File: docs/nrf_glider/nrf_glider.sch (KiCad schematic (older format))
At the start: 26 parts

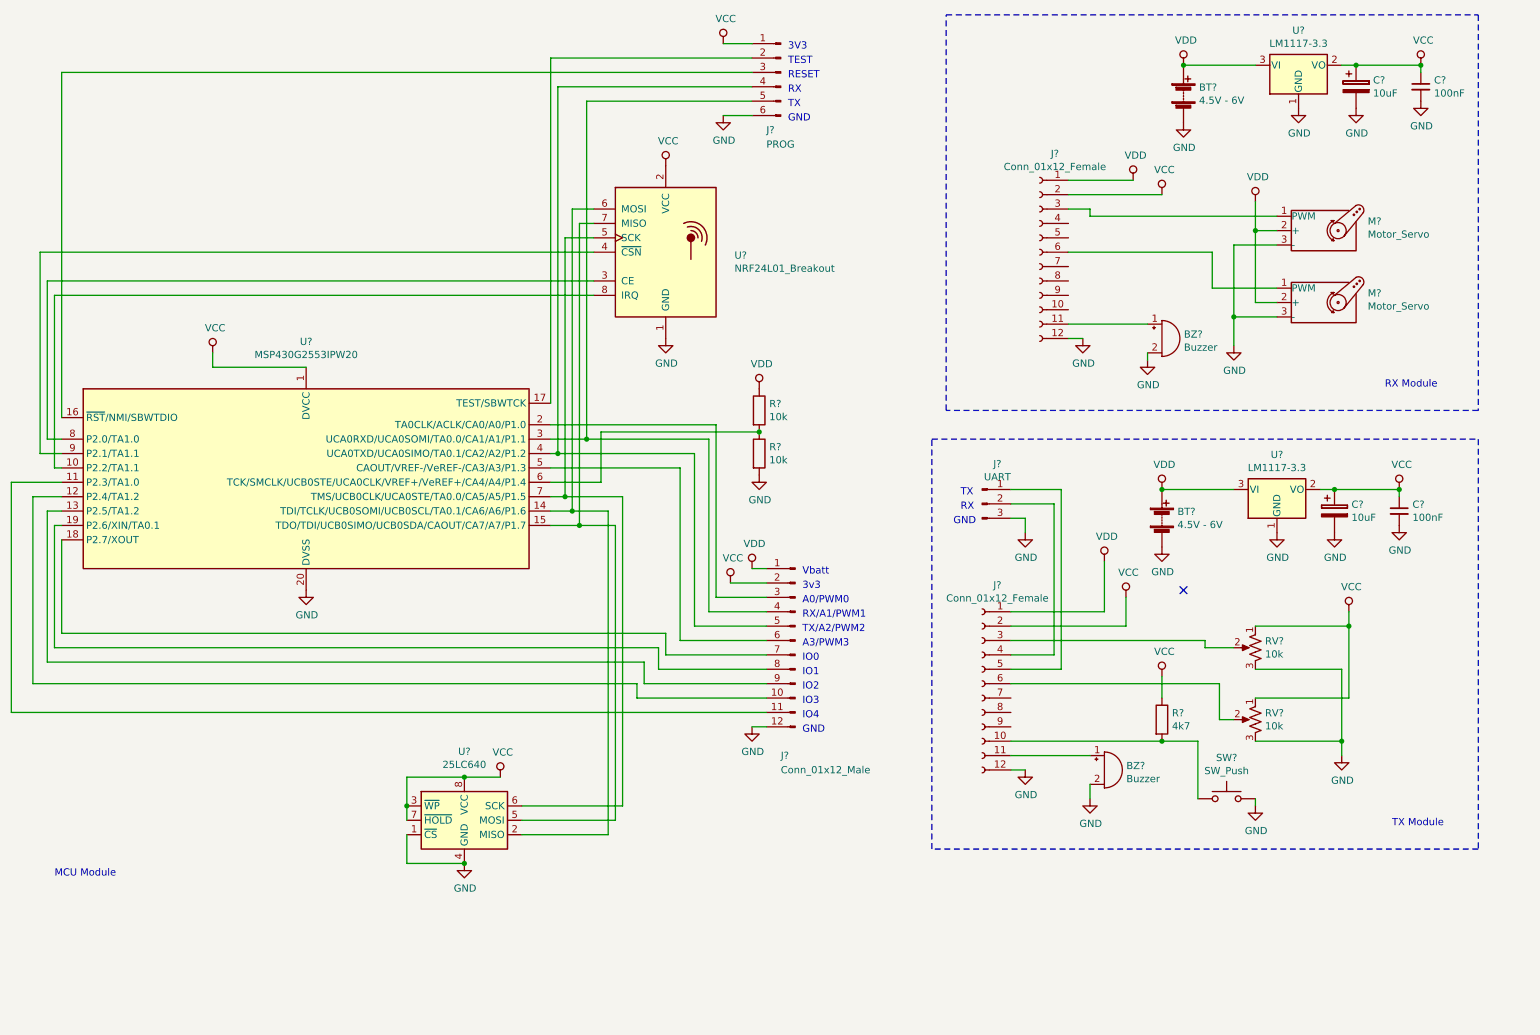
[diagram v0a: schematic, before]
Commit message: tweaks to schematic
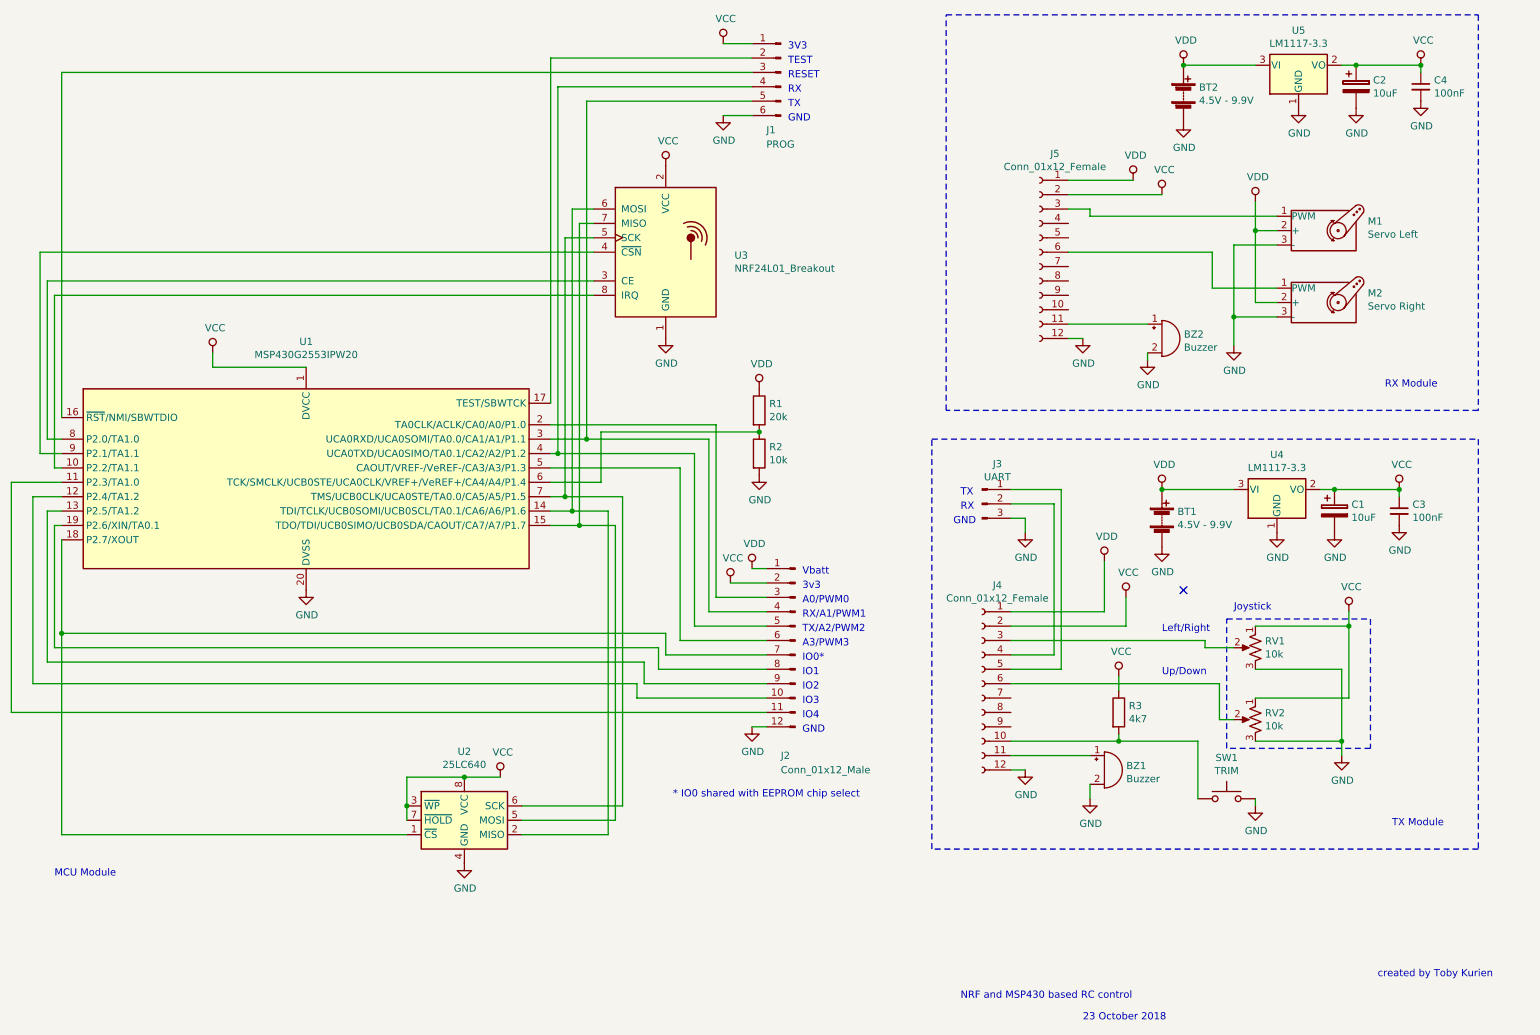
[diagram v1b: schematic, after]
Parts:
- BT1, BT2: renamed from BT?; value 4.5V - 6V -> 4.5V - 9.9V
- M1: renamed from M?; value Motor_Servo -> Servo Left
- M2: renamed from M?; value Motor_Servo -> Servo Right
- R1: renamed from R?; value 10k -> 20k
- SW1: renamed from SW?; value SW_Push -> TRIM
- gave numbers to parts that had none: 20
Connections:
- net GND: no longer U2.1 (~CS)
- net at J2.7 (Pin_7), U1.18 (P2.7/XOUT): now also U2.1 (~CS)
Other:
- note added: "* IO0 shared with EEPROM chip select"
- note added: "23 October 2018"
- note added: "IO0*"
- note added: "Joystick"
- note added: "Left/Right\n"
- note added: "NRF and MSP430 based RC control"
- note added: "Up/Down"
- note added: "created by Toby Kurien"
- note removed: "IO0"
- moved on the sheet: R3

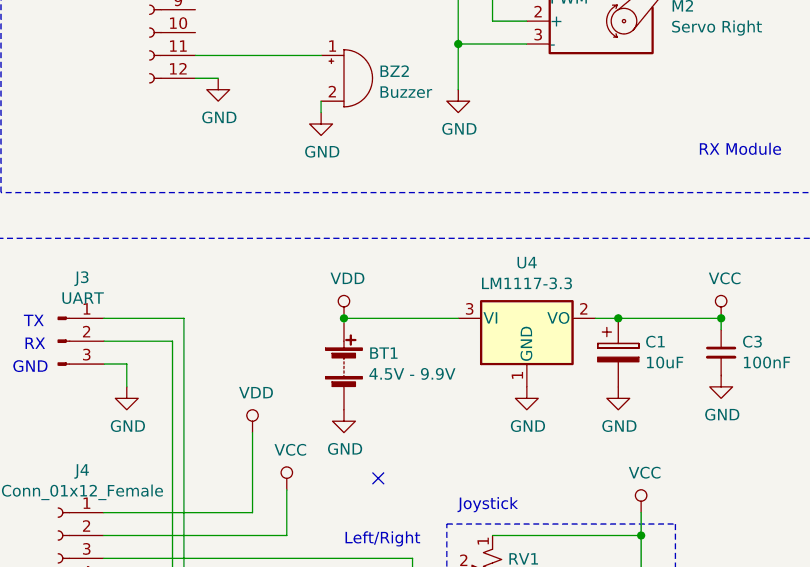
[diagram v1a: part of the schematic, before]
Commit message: added switch
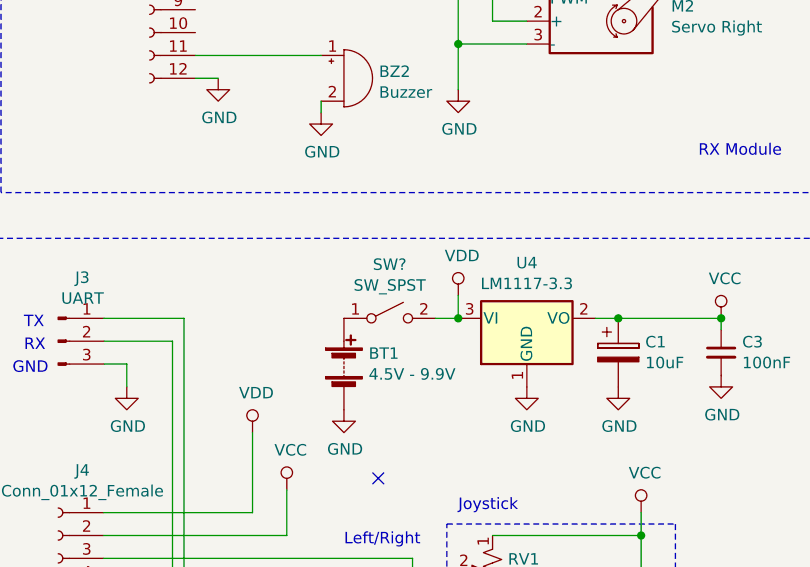
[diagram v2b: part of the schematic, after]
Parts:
- added SW?: SW_SPST, symbol Switch:SW_SPST
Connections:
- net VDD: now also SW?.2 (B); no longer BT1.1 (+)
- new net: BT1.1 (+), SW?.1 (A)
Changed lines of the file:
@@
 	1    0    0    -1
 $EndComp
-Wire Wire Line
-	8800 3950 9300 3950
 $Comp
 L power:GND #PWR025
@@
 L power:VDD #PWR024
 U 1 1 5BD2C8A2
-P 8800 3950
-F 0 "#PWR024" H 8800 3800 50  0001 C CNN
-F 1 "VDD" H 8817 4123 50  0000 C CNN
-F 2 "" H 8800 3950 50  0001 C CNN
-F 3 "" H 8800 3950 50  0001 C CNN
-	1    8800 3950
-	1    0    0    -1
-$EndComp
-Connection ~ 8800 3950
+P 9300 3850
+F 0 "#PWR024" H 9300 3700 50  0001 C CNN
+F 1 "VDD" H 9317 4023 50  0000 C CNN
+F 2 "" H 9300 3850 50  0001 C CNN
+F 3 "" H 9300 3850 50  0001 C CNN
+	1    9300 3850
+	1    0    0    -1
+$EndComp
 Wire Wire Line
 	10450 3950 10450 4000
@@
 	8500 5700 9050 5700
 Wire Wire Line
-	3950 5950 4200 5950
-Wire Wire Line
-	3550 5950 3950 5950
-Connection ~ 3950 5950
-Connection ~ 3550 6150
-Wire Wire Line
-	3550 6150 3550 5950
-Wire Wire Line
-	3550 6250 3550 6150
-Wire Wire Line
 	3550 6350 1150 6350
 Wire Wire Line
@@
 Text Notes 10300 7350 0    50   ~ 0
 created by Toby Kurien
+$Comp
+L Switch:SW_SPST SW?
+U 1 1 5BD0D3D1
+P 9000 3950
+F 0 "SW?" H 9000 4185 50  0000 C CNN
+F 1 "SW_SPST" H 9000 4094 50  0000 C CNN
+F 2 "" H 9000 3950 50  0001 C CNN
+F 3 "" H 9000 3950 50  0001 C CNN
+	1    9000 3950
+	1    0    0    -1
+$EndComp
+Wire Wire Line
+	9200 3950 9300 3950
+Wire Wire Line
+	9300 3850 9300 3950
+Connection ~ 9300 3950
+Wire Wire Line
+	3550 6250 3550 6150
+Wire Wire Line
+	3550 6150 3550 5950
+Connection ~ 3550 6150
+Connection ~ 3950 5950
+Wire Wire Line
+	3550 5950 3950 5950
+Wire Wire Line
+	3950 5950 4200 5950
 $EndSCHEMATC
